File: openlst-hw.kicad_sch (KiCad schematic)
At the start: 8 parts

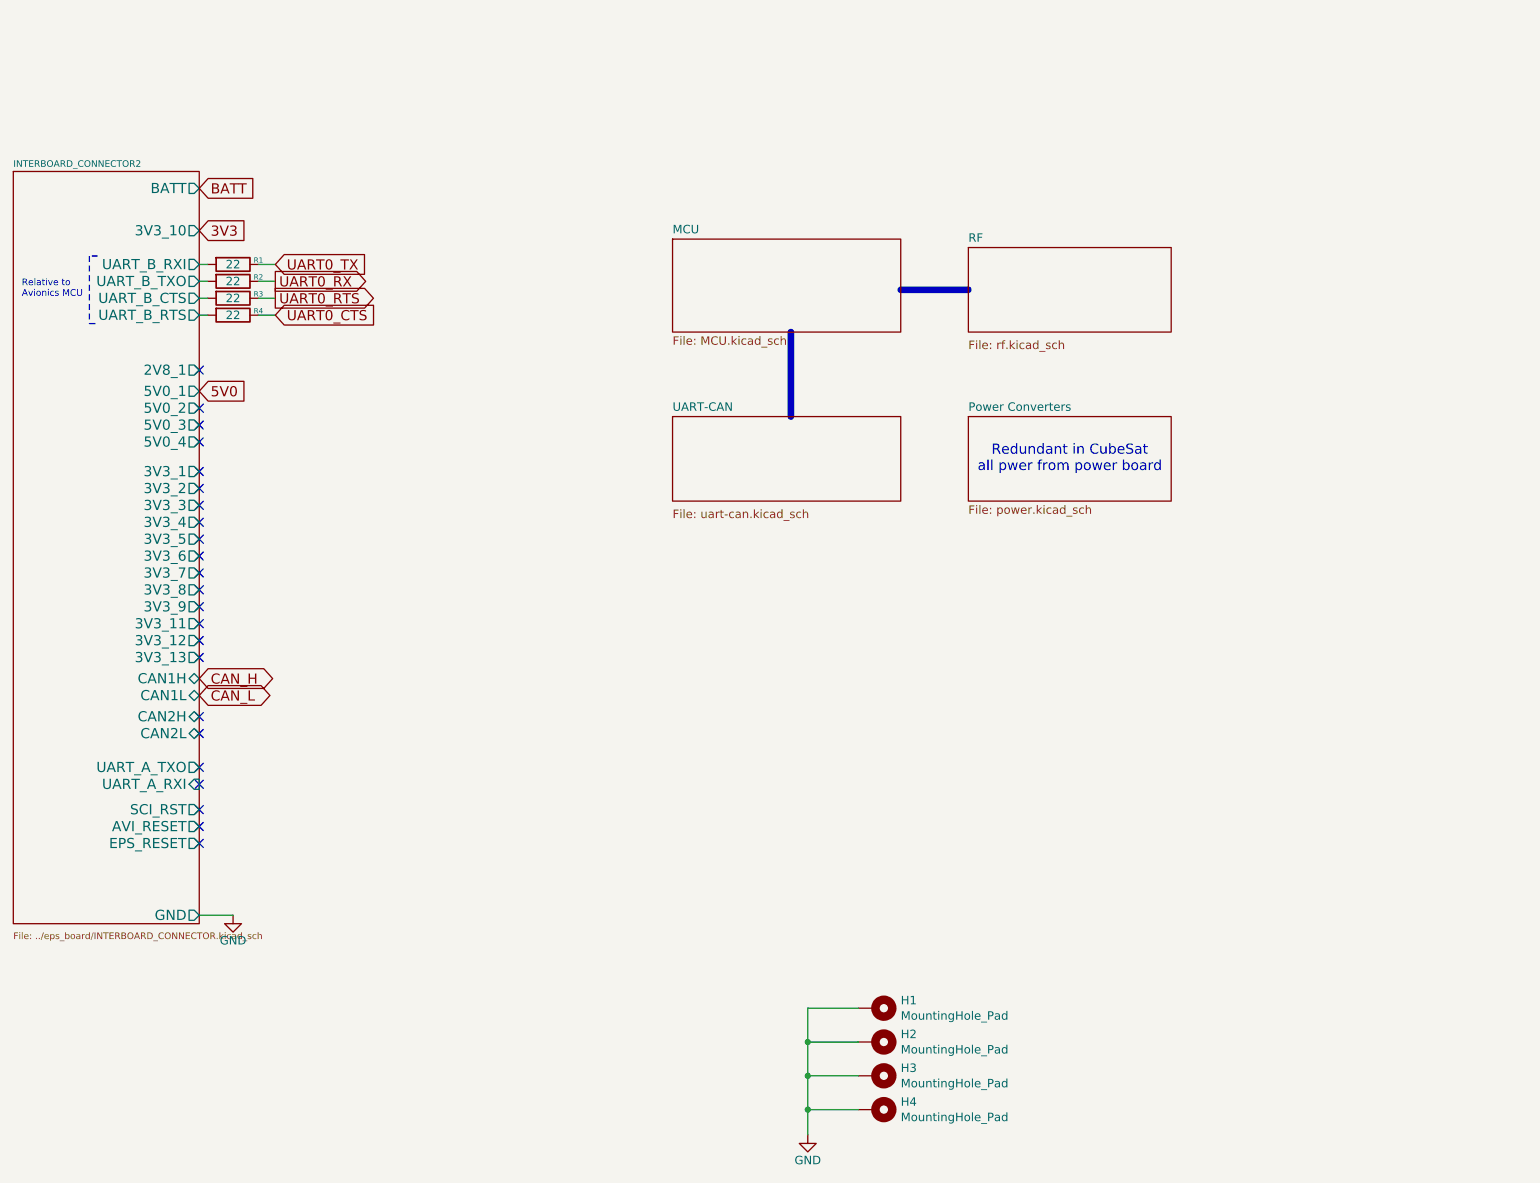
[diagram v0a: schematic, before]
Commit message: temporary branch for radio to pc104
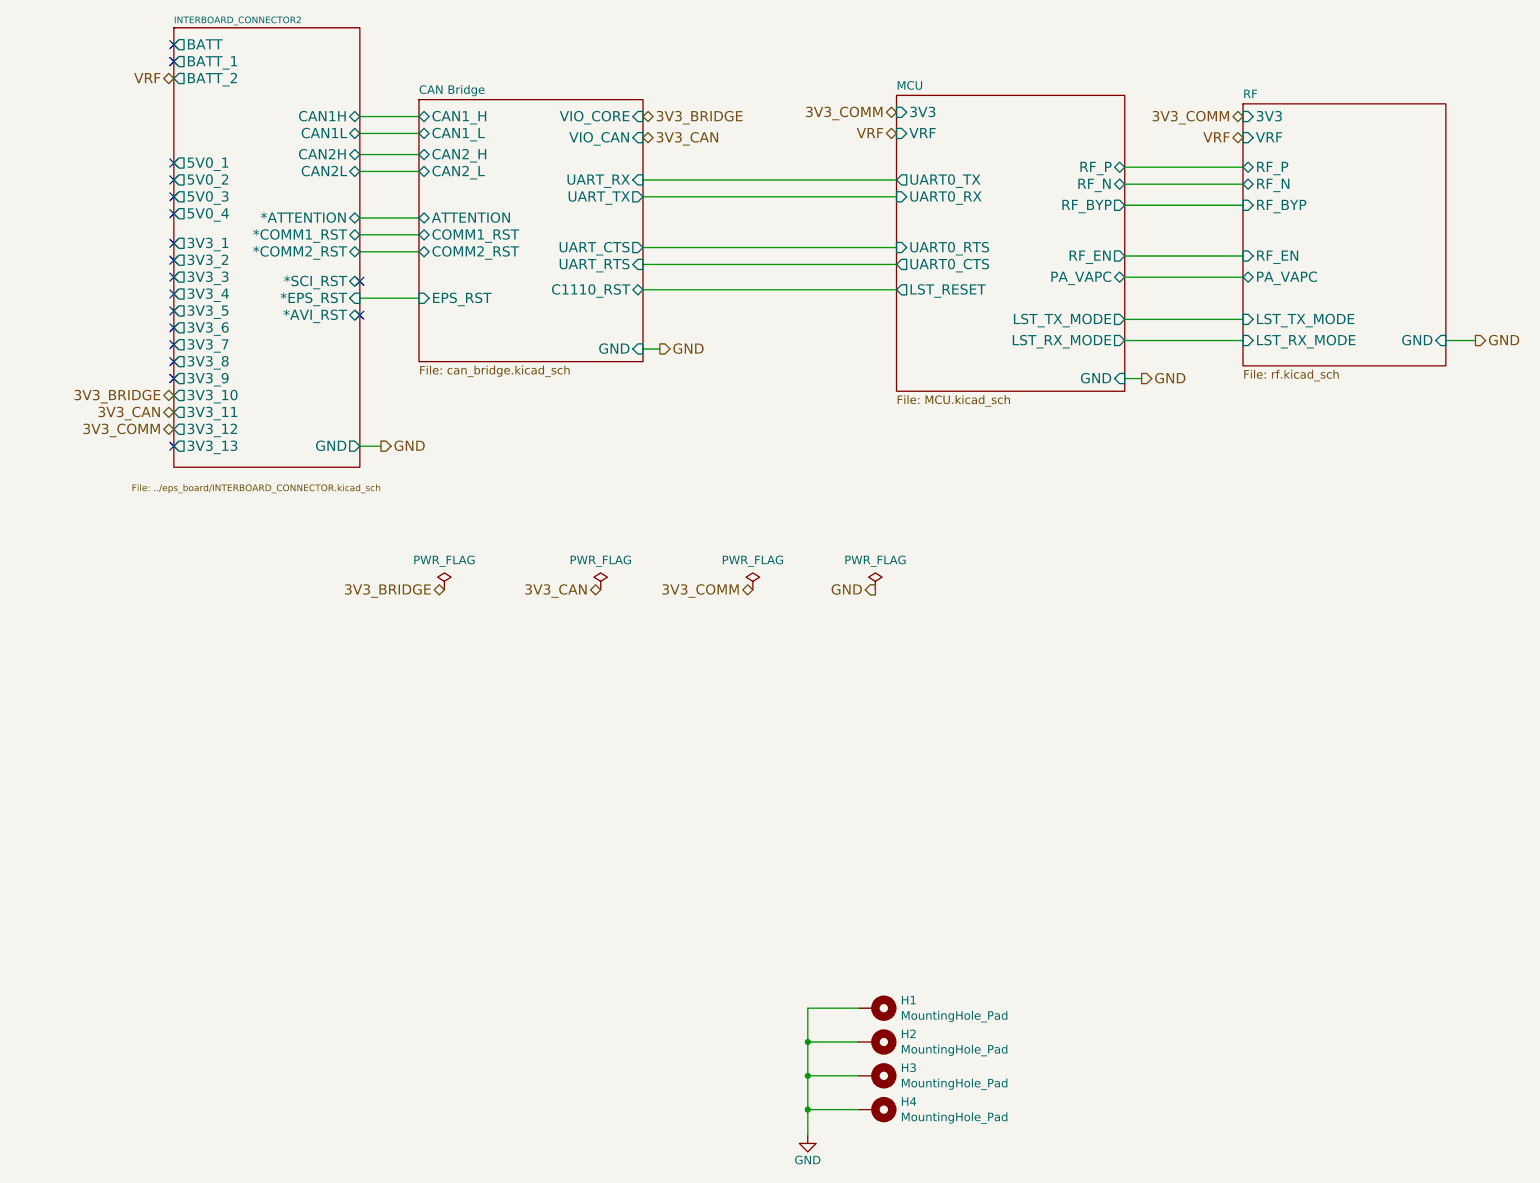
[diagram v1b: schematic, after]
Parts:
- removed R1, R2, R3, R4: 22, Resistor_SMD:R_0603_1608Metric_Pad0.98x0.95mm_HandSolder, symbol Device:R
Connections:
- no-connect marks 23 -> 18
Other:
- removed sheet Power Converters
- removed sheet UART-CAN
- added sheet CAN Bridge (can_bridge.kicad_sch)
- sheet INTERBOARD_CONNECTOR2 ports: added *ATTENTION, *AVI_RST, *COMM1_RST, *COMM2_RST, *EPS_RST, *SCI_RST, BATT_1, BATT_2; removed 2V8_1, AVI_RESET, EPS_RESET, SCI_RST, UART_A_RXI, UART_A_TXO, UART_B_CTS, UART_B_RTS, UART_B_RXI, UART_B_TXO
- sheet MCU ports: added 3V3, GND, LST_RESET, LST_RX_MODE, LST_TX_MODE, PA_VAPC, RF_BYP, RF_EN, RF_N, RF_P, UART0_CTS, UART0_RTS, UART0_RX, UART0_TX, VRF; removed none
- sheet RF ports: added 3V3, GND, LST_RX_MODE, LST_TX_MODE, PA_VAPC, RF_BYP, RF_EN, RF_N, RF_P, VRF; removed none
- note removed: "Redundant in CubeSat all pwer from power board"
- note removed: "Relative to Avionics MCU"
